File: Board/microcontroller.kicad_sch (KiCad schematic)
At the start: 22 parts, among them J9 ICSP, U2 PIC18F2480-ISO, Y1 10 MHz

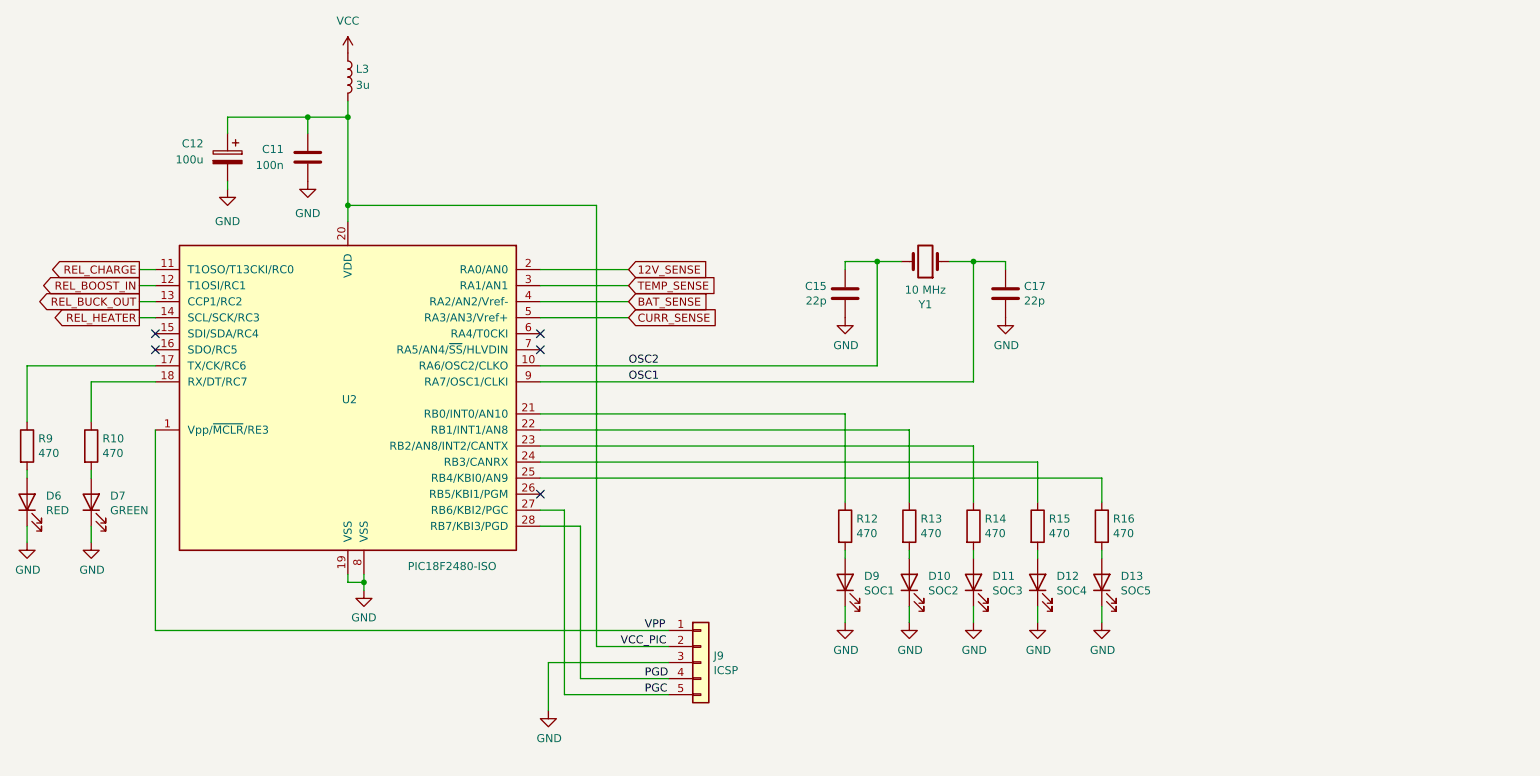
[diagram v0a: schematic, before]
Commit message: Rev 1.0
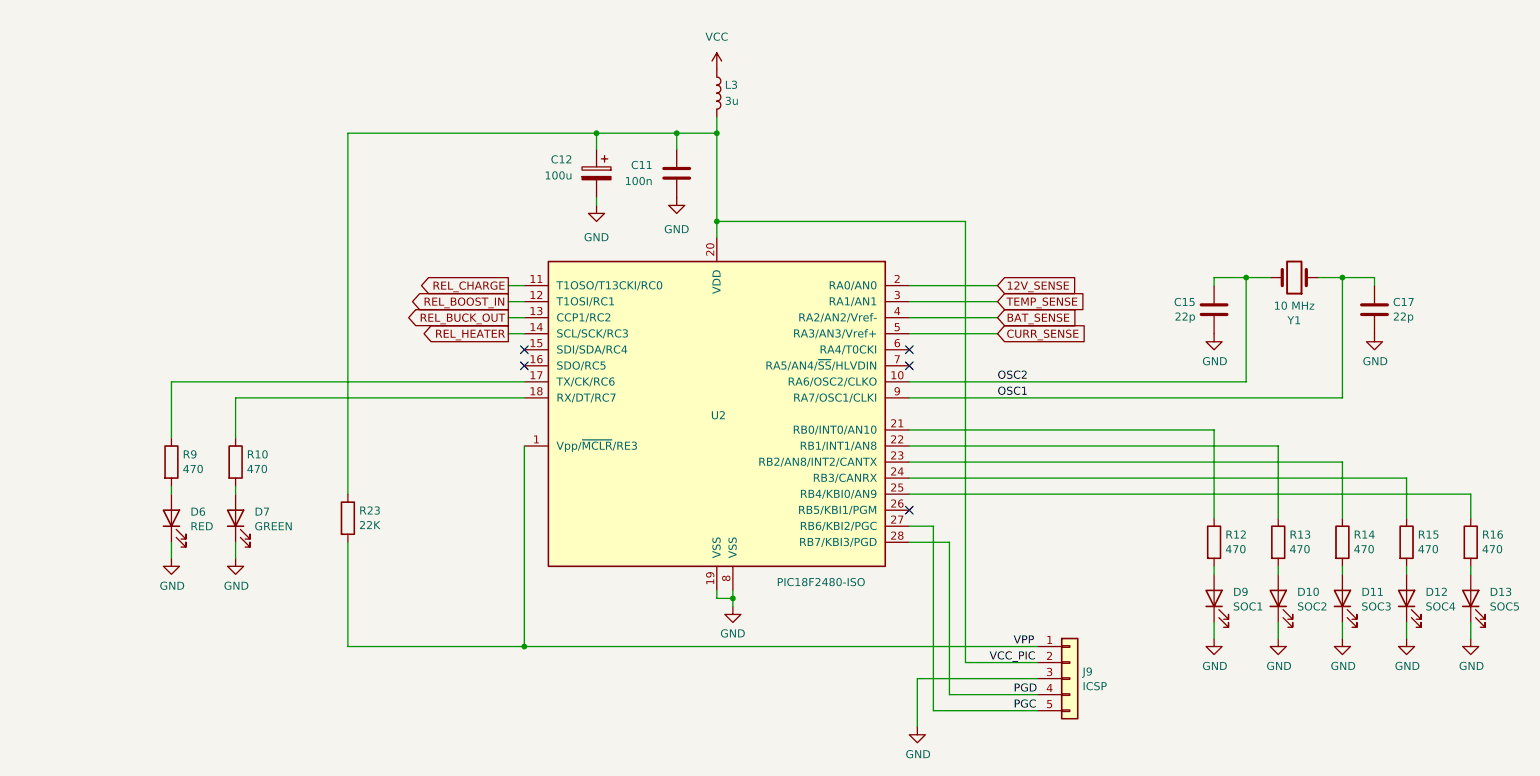
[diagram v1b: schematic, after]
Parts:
- added R23: 22K, Resistor_SMD:R_0805_2012Metric, symbol Device:R
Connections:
- net VCC_PIC: now also R23.1
- net VPP: now also R23.2
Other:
- moved on the sheet: C11, C12, C15, C17, D10, D11, D12, D13, D6, D7, D9, J9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

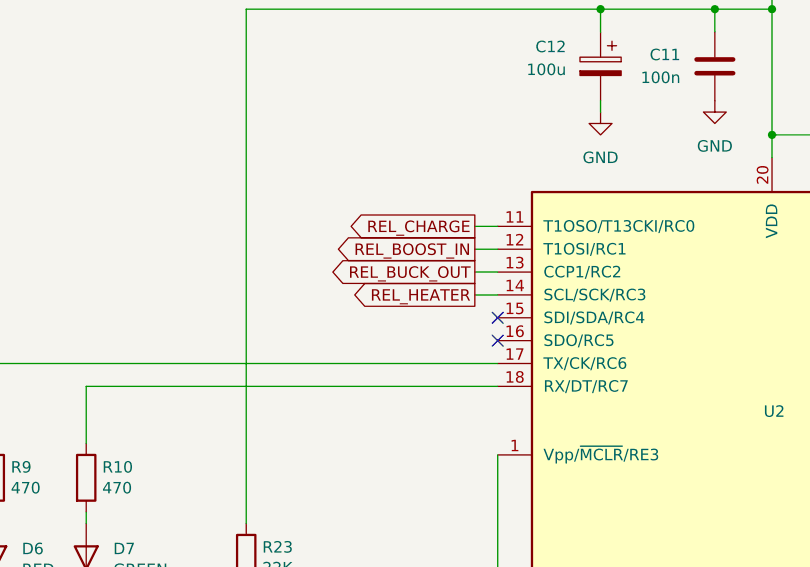
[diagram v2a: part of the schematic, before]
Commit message: WIP
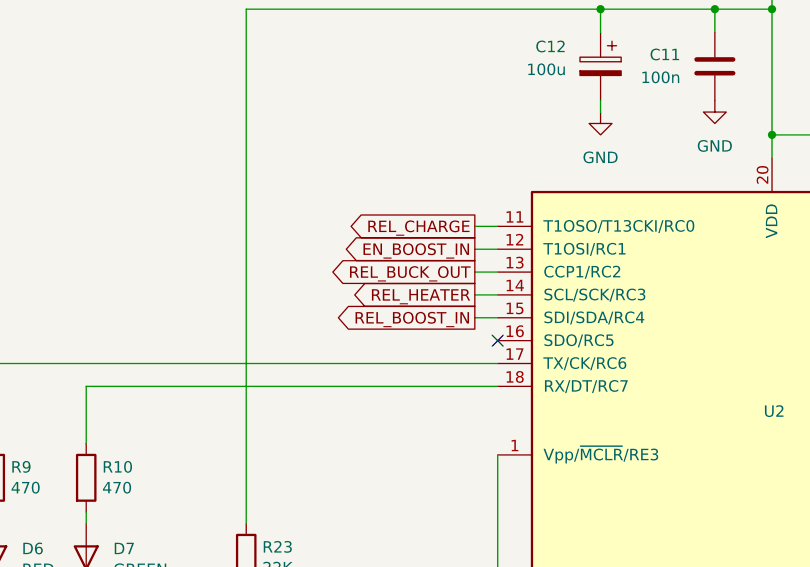
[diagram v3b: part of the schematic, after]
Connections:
- net REL_BOOST_IN: now also U2.15 (SDI/SDA/RC4); no longer U2.12 (T1OSI/RC1)
- new net EN_BOOST_IN: U2.12 (T1OSI/RC1)
- no-connect marks 5 -> 4
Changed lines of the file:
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@@
-	)
-	(no_connect
-		(at 107.95 80.01)
 	)
 	(no_connect
@@
 		(pts
 			(xy 175.26 134.62) (xy 175.26 110.49)
+		)
+		(stroke
+			(width 0)
+			(type default)
+		)
+	)
+	(wire
+		(pts
+			(xy 105.41 80.01) (xy 107.95 80.01)
 		)
 		(stroke
@@
 		)
 	)
-	(global_label "REL_BOOST_IN"
+	(global_label "EN_BOOST_IN"
 		(shape output)
 		(at 105.41 72.39 180)
@@
 		)
 		(property "Intersheetrefs" "${INTERSHEET_REFS}"
-			(at 88.9991 72.39 0)
+			(at 89.9667 72.39 0)
 			(effects
 				(font
@@
 				(hide yes)
 			)
+		)
+	)
+	(global_label "REL_BOOST_IN"
+		(shape output)
+		(at 105.41 80.01 180)
+		(fields_autoplaced yes)
+		(effects
+			(font
+				(size 1.27 1.27)
+			)
+			(justify right)
+		)
+		(property "Intersheetrefs" "${INTERSHEET_REFS}"
+			(at 88.9991 80.01 0)
+			(effects
+				(font
+					(size 1.27 1.27)
+				)
+				(justify right)
+				(hide yes)
+			)
